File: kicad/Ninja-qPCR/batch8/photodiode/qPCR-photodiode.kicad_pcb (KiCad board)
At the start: 2 copper layers, 104.1 x 42 mm, 34 parts, among them J1 Conn_01x20_Male, J2 Conn_01x20_Male

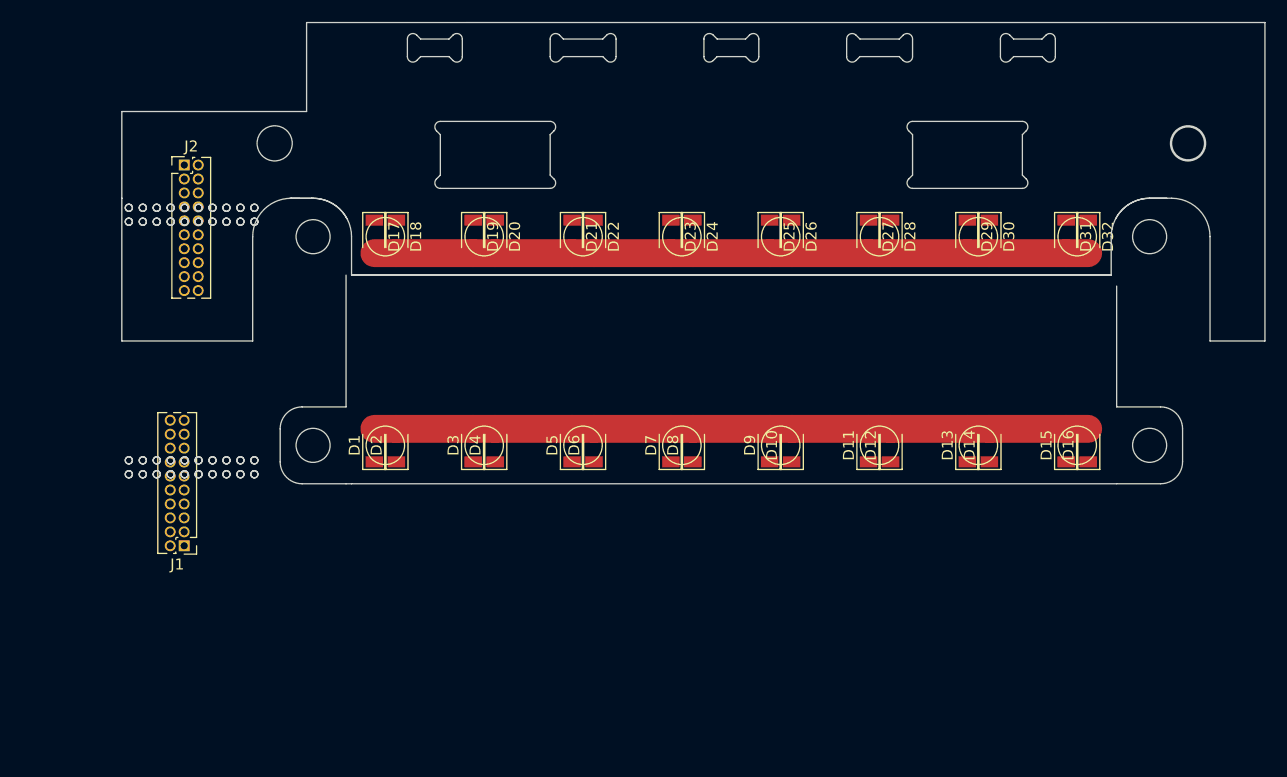
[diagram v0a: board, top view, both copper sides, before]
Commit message: order batch8
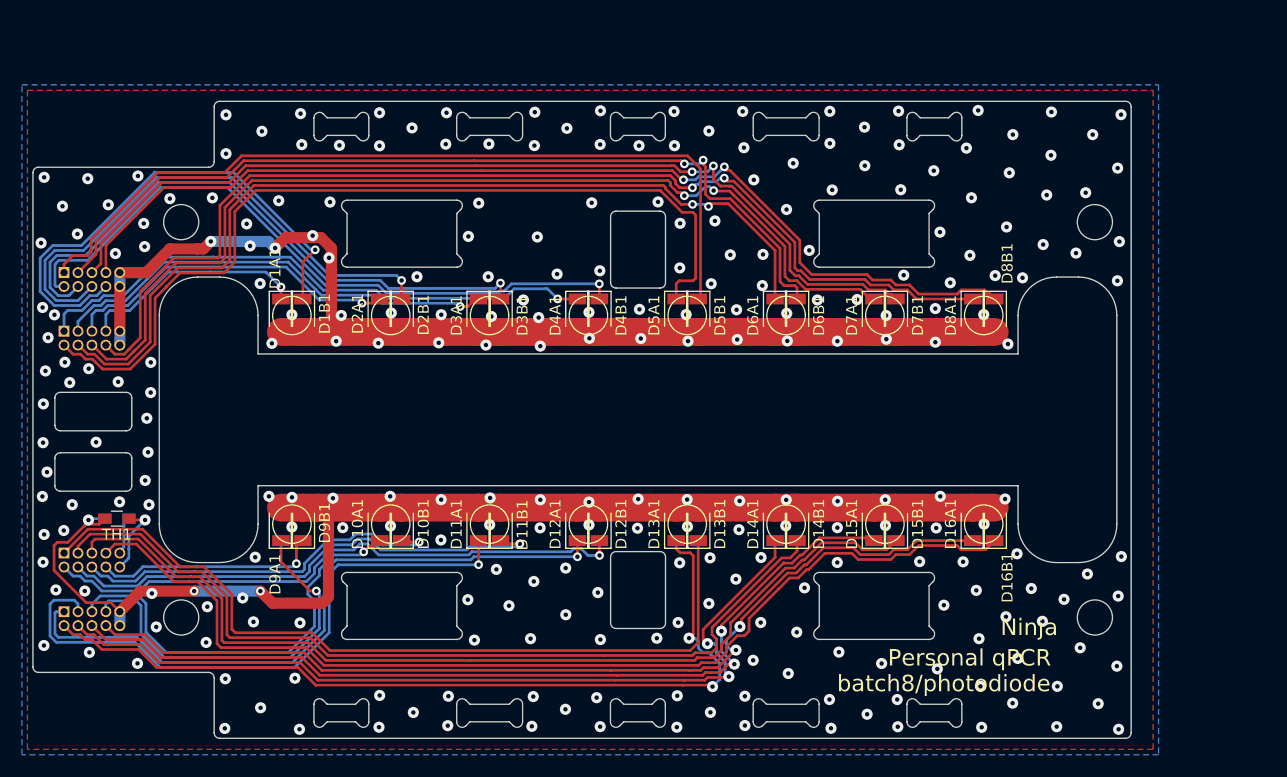
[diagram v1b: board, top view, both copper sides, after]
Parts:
- removed D1, D10, D11, D12, D13, D14, D15, D16, D17, D2, D3, D4, D5, D6, D7, D8, D9: D_Photo, Diodes_SMD:D_1206
- removed J1, J2: Conn_01x20_Male, Pin_Headers:Pin_Header_Straight_2x10_Pitch1.27mm
- added D10A1: D_Photo, Diodes_SMD:D_1206, F.Cu at (114.6, 109.5)
- added D10B1: D_Photo, Diodes_SMD:D_1206, F.Cu at (116.6, 109.5)
- added D11A1: D_Photo, Diodes_SMD:D_1206, F.Cu at (123.6, 109.5)
- added D11B1: D_Photo, Diodes_SMD:D_1206, F.Cu at (125.6, 109.5)
- added D12A1: D_Photo, Diodes_SMD:D_1206, F.Cu at (132.6, 109.5)
- added D12B1: D_Photo, Diodes_SMD:D_1206, F.Cu at (134.6, 109.5)
- added D13A1: D_Photo, Diodes_SMD:D_1206, F.Cu at (141.6, 109.5)
- added D13B1: D_Photo, Diodes_SMD:D_1206, F.Cu at (143.6, 109.5)
- added D14A1: D_Photo, Diodes_SMD:D_1206, F.Cu at (150.6, 109.5)
- added D14B1: D_Photo, Diodes_SMD:D_1206, F.Cu at (152.6, 109.5)
- added D15A1: D_Photo, Diodes_SMD:D_1206, F.Cu at (159.6, 109.5)
- added D15B1: D_Photo, Diodes_SMD:D_1206, F.Cu at (161.6, 109.5)
- added D16A1: D_Photo, Diodes_SMD:D_1206, F.Cu at (168.6, 109.5)
- added D16B1: D_Photo, Diodes_SMD:D_1206, F.Cu at (170.6, 109.5)
- added D1A1: D_Photo, Diodes_SMD:D_1206, F.Cu at (105.6, 90.5)
- added D9A1: D_Photo, Diodes_SMD:D_1206, F.Cu at (105.6, 109.5)
- added D9B1: D_Photo, Diodes_SMD:D_1206, F.Cu at (107.6, 109.5)
- added JNA1: Conn_01x10_Male, Pin_Headers:Pin_Header_Straight_2x05_Pitch1.27mm, B.Cu at (85.8, 91.9)
- added JNB1: Conn_01x10_Male, Pin_Headers:Pin_Header_Straight_2x05_Pitch1.27mm, B.Cu at (85.8, 86.6)
- added JSA1: Conn_01x10_Male, Pin_Headers:Pin_Header_Straight_2x05_Pitch1.27mm, B.Cu at (85.8, 117.5)
- added JSB1: Conn_01x10_Male, Pin_Headers:Pin_Header_Straight_2x05_Pitch1.27mm, B.Cu at (85.8, 112.1)
- added TH1: Thermistor, Resistors_SMD:R_0603_HandSoldering, F.Cu at (90.6, 109.0)
- added TH2: Thermistor, Resistors_SMD:R_0603_HandSoldering, B.Cu at (90.6, 109.0)
- moved D1B1 11.1 mm to (107.6, 90.5)
- moved D2A1 11.1 mm to (114.6, 90.5)
- moved D2B1 11.1 mm to (116.6, 90.5)
- moved D3A1 11.1 mm to (123.6, 90.5)
- moved D3B1 11.1 mm to (125.6, 90.5)
- moved D4A1 11.1 mm to (132.6, 90.5)
- moved D4B1 11.1 mm to (134.6, 90.5)
- moved D5A1 11.1 mm to (141.6, 90.5)
- moved D5B1 11.1 mm to (143.6, 90.5)
- moved D6A1 11.1 mm to (150.6, 90.5)
- moved D6B1 11.1 mm to (152.6, 90.5)
- moved D7A1 11.1 mm to (159.6, 90.5)
- moved D7B1 11.1 mm to (161.6, 90.5)
- moved D8A1 11.1 mm to (168.6, 90.5)
- moved D8B1 11.1 mm to (170.6, 90.5)
- renumbered D18 to D1B1, D19 to D2A1, D20 to D2B1, D21 to D3A1, D22 to D3B1, D23 to D4A1, D24 to D4B1, D25 to D5A1, D26 to D5B1, D27 to D6A1, D28 to D6B1, D29 to D7A1, D30 to D7B1, D31 to D8A1, D32 to D8B1
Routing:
- net /N_PD_OUT15: track 0.00 -> 98.5 mm, vias 0 -> 2
- net /S_PD_OUT16: track 0.00 -> 94.9 mm
- net /N_PD_OUT16: track 0.00 -> 93.8 mm, vias 0 -> 2
- net /N_PD_OUT13: track 0.00 -> 90.8 mm, vias 0 -> 2
- net /S_PD_OUT15: track 0.00 -> 88.4 mm, vias 0 -> 2
- net /S_PD_OUT14: track 0.00 -> 87.1 mm
- net /N_PD_OUT14: track 0.00 -> 86.0 mm, vias 0 -> 2
- net GNDA: track 130.0 -> 213.7 mm, vias 0 -> 273
- net /N_PD_OUT11: track 0.00 -> 83.3 mm, vias 0 -> 2
- net /S_PD_OUT13: track 0.00 -> 82.1 mm, vias 0 -> 2
- net /N_PD_OUT9: track 0.00 -> 80.4 mm
- net /N_PD_OUT12: track 0.00 -> 80.0 mm, vias 0 -> 2
- net /S_PD_OUT12: track 0.00 -> 79.8 mm
- net /S_PD_OUT9: track 0.00 -> 78.0 mm, vias 0 -> 2
- net /S_PD_OUT11: track 0.00 -> 78.0 mm, vias 0 -> 2
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- added copper zone on B.Cu, net GNDA
- added copper zone on F.Cu, net GNDA
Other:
- board size 104.1 x 42 mm -> 100 x 58 mm
- board text added: "100x58mm"
- board text added: "Ninja"
- board text added: "Personal qPCR"
- board text added: "batch8/photodiode"
